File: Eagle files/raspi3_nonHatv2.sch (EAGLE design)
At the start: 37 parts, among them IC5 PAM8403, K1 PIN20X2

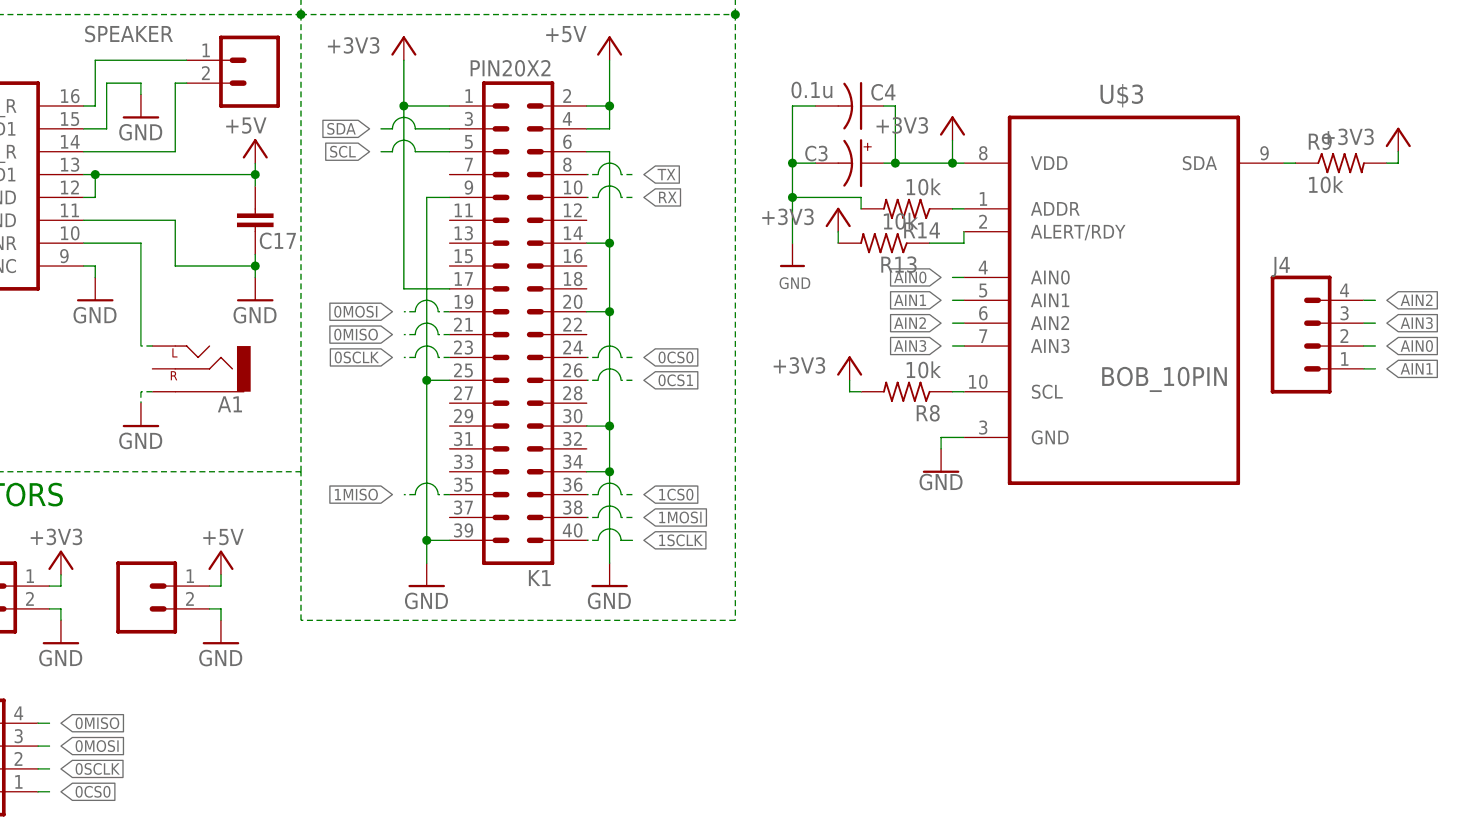
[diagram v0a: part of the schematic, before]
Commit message: rearranged
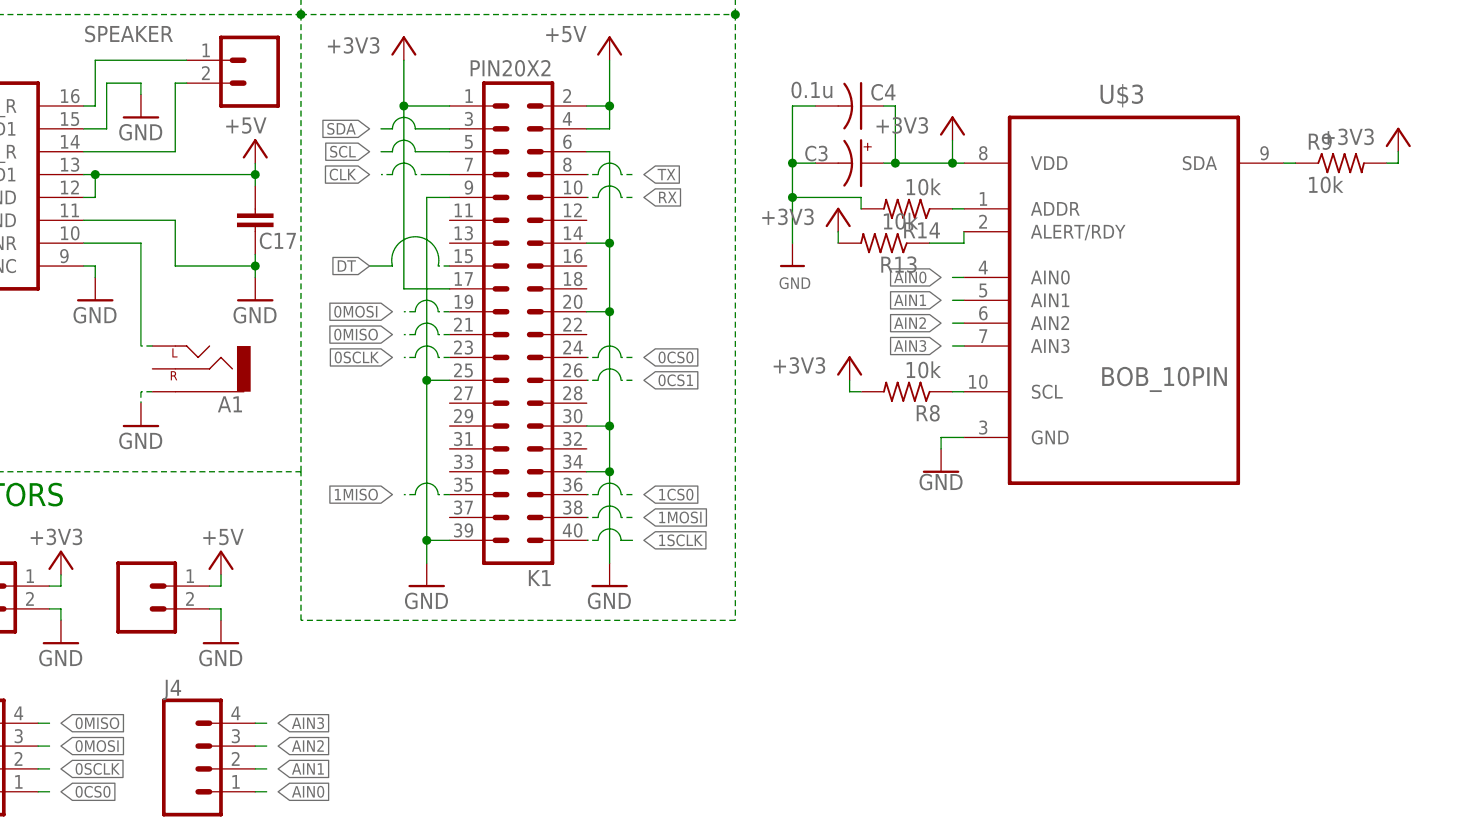
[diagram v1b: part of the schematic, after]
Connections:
- net AIN0: now also J4.1; no longer J4.2
- net AIN1: now also J4.2; no longer J4.1
- net AIN2: now also J4.3; no longer J4.4
- net AIN3: now also J4.4; no longer J4.3
- net CLK: now also K1.7
- net DT: now also K1.15
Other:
- moved on the sheet: J4
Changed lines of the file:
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@@
 <?xml version="1.0" encoding="utf-8"?>
 <!DOCTYPE eagle SYSTEM "eagle.dtd">
-<eagle version="9.6.2">
+<eagle version="9.4.1">
 <drawing>
 <settings>
@@
 <attribute name="NAME" x="-19.05" y="5.588" size="1.778" layer="95" font="vector"/>
 </instance>
-<instance part="J4" gate="G$1" x="133.35" y="44.45" smashed="yes">
-<attribute name="VALUE" x="128.27" y="37.084" size="1.778" layer="96" font="vector"/>
-<attribute name="NAME" x="128.27" y="52.578" size="1.778" layer="95" font="vector"/>
+<instance part="J4" gate="G$1" x="10.16" y="-2.54" smashed="yes">
+<attribute name="VALUE" x="5.08" y="-9.906" size="1.778" layer="96" font="vector"/>
+<attribute name="NAME" x="5.08" y="5.588" size="1.778" layer="95" font="vector"/>
 </instance>
 <instance part="U$3" gate="G$1" x="111.76" y="49.53" smashed="yes">
@@
 <label x="-34.29" y="119.38" size="1.27" layer="95" font="vector" ratio="17" rot="R90" xref="yes"/>
 </segment>
+<segment>
+<wire x1="36.83" y1="53.34" x2="35.56" y2="53.34" width="0.1524" layer="91" style="dashdot"/>
+<pinref part="K1" gate="G$1" pin="15"/>
+<wire x1="35.56" y1="53.34" x2="30.48" y2="53.34" width="0.1524" layer="91" curve="208.072487"/>
+<wire x1="30.48" y1="53.34" x2="27.94" y2="53.34" width="0.1524" layer="91"/>
+<label x="27.94" y="53.34" size="1.27" layer="95" font="vector" ratio="16" rot="R180" xref="yes"/>
+</segment>
 </net>
 <net name="CLK" class="0">
@@
 <wire x1="-41.91" y1="118.11" x2="-41.91" y2="115.57" width="0.1524" layer="91"/>
 <label x="-41.91" y="119.38" size="1.27" layer="95" font="vector" ratio="17" rot="R90" xref="yes"/>
+</segment>
+<segment>
+<wire x1="34.29" y1="63.5" x2="33.02" y2="63.5" width="0.1524" layer="91" style="dashdot"/>
+<wire x1="33.02" y1="63.5" x2="30.48" y2="63.5" width="0.1524" layer="91" curve="180"/>
+<wire x1="30.48" y1="63.5" x2="29.21" y2="63.5" width="0.1524" layer="91" style="dashdot"/>
+<pinref part="K1" gate="G$1" pin="7"/>
+<wire x1="36.83" y1="63.5" x2="34.29" y2="63.5" width="0.1524" layer="91"/>
+<label x="27.94" y="63.5" size="1.27" layer="95" font="vector" ratio="16" rot="R180" xref="yes"/>
 </segment>
 </net>
@@
 </segment>
 <segment>
-<pinref part="J4" gate="G$1" pin="2"/>
-<wire x1="138.43" y1="44.45" x2="139.7" y2="44.45" width="0.1524" layer="91"/>
-<label x="140.97" y="44.45" size="1.27" layer="95" font="vector" ratio="16" xref="yes"/>
+<pinref part="J4" gate="G$1" pin="1"/>
+<wire x1="15.24" y1="-5.08" x2="16.51" y2="-5.08" width="0.1524" layer="91"/>
+<label x="17.78" y="-5.08" size="1.27" layer="95" font="vector" ratio="16" xref="yes"/>
 </segment>
 </net>
@@
 </segment>
 <segment>
-<pinref part="J4" gate="G$1" pin="1"/>
-<wire x1="138.43" y1="41.91" x2="139.7" y2="41.91" width="0.1524" layer="91"/>
-<label x="140.97" y="41.91" size="1.27" layer="95" font="vector" ratio="16" xref="yes"/>
+<pinref part="J4" gate="G$1" pin="2"/>
+<wire x1="15.24" y1="-2.54" x2="16.51" y2="-2.54" width="0.1524" layer="91"/>
+<label x="17.78" y="-2.54" size="1.27" layer="95" font="vector" ratio="16" xref="yes"/>
 </segment>
 </net>
@@
 </segment>
 <segment>
-<pinref part="J4" gate="G$1" pin="4"/>
-<wire x1="138.43" y1="49.53" x2="139.7" y2="49.53" width="0.1524" layer="91"/>
-<label x="140.97" y="49.53" size="1.27" layer="95" font="vector" ratio="16" xref="yes"/>
+<pinref part="J4" gate="G$1" pin="3"/>
+<wire x1="15.24" y1="0" x2="16.51" y2="0" width="0.1524" layer="91"/>
+<label x="17.78" y="0" size="1.27" layer="95" font="vector" ratio="16" xref="yes"/>
 </segment>
 </net>
@@
 </segment>
 <segment>
-<pinref part="J4" gate="G$1" pin="3"/>
-<wire x1="138.43" y1="46.99" x2="139.7" y2="46.99" width="0.1524" layer="91"/>
-<label x="140.97" y="46.99" size="1.27" layer="95" font="vector" ratio="16" xref="yes"/>
-</segment>
-</net>
+<pinref part="J4" gate="G$1" pin="4"/>
+<wire x1="15.24" y1="2.54" x2="16.51" y2="2.54" width="0.1524" layer="91"/>
+<label x="17.78" y="2.54" size="1.27" layer="95" font="vector" ratio="16" xref="yes"/>
+</segment>
+</net>

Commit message: restored v4
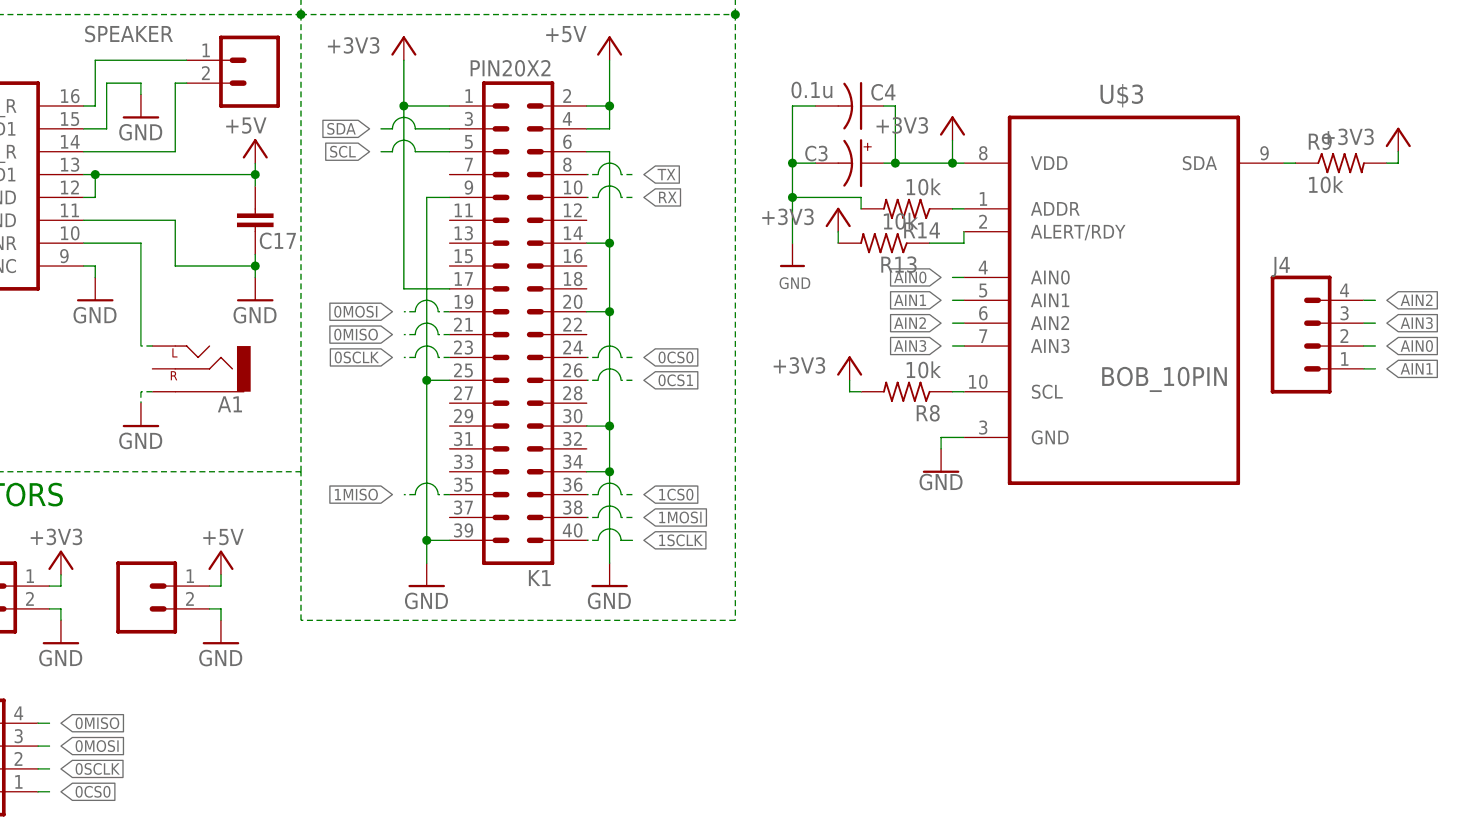
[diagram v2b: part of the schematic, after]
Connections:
- net AIN0: now also J4.2; no longer J4.1
- net AIN1: now also J4.1; no longer J4.2
- net AIN2: now also J4.4; no longer J4.3
- net AIN3: now also J4.3; no longer J4.4
- net CLK: no longer K1.7
- net DT: no longer K1.15
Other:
- moved on the sheet: J4
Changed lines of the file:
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@@
 <?xml version="1.0" encoding="utf-8"?>
 <!DOCTYPE eagle SYSTEM "eagle.dtd">
-<eagle version="9.4.1">
+<eagle version="9.6.2">
 <drawing>
 <settings>
@@
 <attribute name="NAME" x="-19.05" y="5.588" size="1.778" layer="95" font="vector"/>
 </instance>
-<instance part="J4" gate="G$1" x="10.16" y="-2.54" smashed="yes">
-<attribute name="VALUE" x="5.08" y="-9.906" size="1.778" layer="96" font="vector"/>
-<attribute name="NAME" x="5.08" y="5.588" size="1.778" layer="95" font="vector"/>
+<instance part="J4" gate="G$1" x="133.35" y="44.45" smashed="yes">
+<attribute name="VALUE" x="128.27" y="37.084" size="1.778" layer="96" font="vector"/>
+<attribute name="NAME" x="128.27" y="52.578" size="1.778" layer="95" font="vector"/>
 </instance>
 <instance part="U$3" gate="G$1" x="111.76" y="49.53" smashed="yes">
@@
 <label x="-34.29" y="119.38" size="1.27" layer="95" font="vector" ratio="17" rot="R90" xref="yes"/>
 </segment>
-<segment>
-<wire x1="36.83" y1="53.34" x2="35.56" y2="53.34" width="0.1524" layer="91" style="dashdot"/>
-<pinref part="K1" gate="G$1" pin="15"/>
-<wire x1="35.56" y1="53.34" x2="30.48" y2="53.34" width="0.1524" layer="91" curve="208.072487"/>
-<wire x1="30.48" y1="53.34" x2="27.94" y2="53.34" width="0.1524" layer="91"/>
-<label x="27.94" y="53.34" size="1.27" layer="95" font="vector" ratio="16" rot="R180" xref="yes"/>
-</segment>
 </net>
 <net name="CLK" class="0">
@@
 <wire x1="-41.91" y1="118.11" x2="-41.91" y2="115.57" width="0.1524" layer="91"/>
 <label x="-41.91" y="119.38" size="1.27" layer="95" font="vector" ratio="17" rot="R90" xref="yes"/>
-</segment>
-<segment>
-<wire x1="34.29" y1="63.5" x2="33.02" y2="63.5" width="0.1524" layer="91" style="dashdot"/>
-<wire x1="33.02" y1="63.5" x2="30.48" y2="63.5" width="0.1524" layer="91" curve="180"/>
-<wire x1="30.48" y1="63.5" x2="29.21" y2="63.5" width="0.1524" layer="91" style="dashdot"/>
-<pinref part="K1" gate="G$1" pin="7"/>
-<wire x1="36.83" y1="63.5" x2="34.29" y2="63.5" width="0.1524" layer="91"/>
-<label x="27.94" y="63.5" size="1.27" layer="95" font="vector" ratio="16" rot="R180" xref="yes"/>
 </segment>
 </net>
@@
 </segment>
 <segment>
-<pinref part="J4" gate="G$1" pin="1"/>
-<wire x1="15.24" y1="-5.08" x2="16.51" y2="-5.08" width="0.1524" layer="91"/>
-<label x="17.78" y="-5.08" size="1.27" layer="95" font="vector" ratio="16" xref="yes"/>
+<pinref part="J4" gate="G$1" pin="2"/>
+<wire x1="138.43" y1="44.45" x2="139.7" y2="44.45" width="0.1524" layer="91"/>
+<label x="140.97" y="44.45" size="1.27" layer="95" font="vector" ratio="16" xref="yes"/>
 </segment>
 </net>
@@
 </segment>
 <segment>
-<pinref part="J4" gate="G$1" pin="2"/>
-<wire x1="15.24" y1="-2.54" x2="16.51" y2="-2.54" width="0.1524" layer="91"/>
-<label x="17.78" y="-2.54" size="1.27" layer="95" font="vector" ratio="16" xref="yes"/>
+<pinref part="J4" gate="G$1" pin="1"/>
+<wire x1="138.43" y1="41.91" x2="139.7" y2="41.91" width="0.1524" layer="91"/>
+<label x="140.97" y="41.91" size="1.27" layer="95" font="vector" ratio="16" xref="yes"/>
 </segment>
 </net>
@@
 </segment>
 <segment>
-<pinref part="J4" gate="G$1" pin="3"/>
-<wire x1="15.24" y1="0" x2="16.51" y2="0" width="0.1524" layer="91"/>
-<label x="17.78" y="0" size="1.27" layer="95" font="vector" ratio="16" xref="yes"/>
+<pinref part="J4" gate="G$1" pin="4"/>
+<wire x1="138.43" y1="49.53" x2="139.7" y2="49.53" width="0.1524" layer="91"/>
+<label x="140.97" y="49.53" size="1.27" layer="95" font="vector" ratio="16" xref="yes"/>
 </segment>
 </net>
@@
 </segment>
 <segment>
-<pinref part="J4" gate="G$1" pin="4"/>
-<wire x1="15.24" y1="2.54" x2="16.51" y2="2.54" width="0.1524" layer="91"/>
-<label x="17.78" y="2.54" size="1.27" layer="95" font="vector" ratio="16" xref="yes"/>
-</segment>
-</net>
+<pinref part="J4" gate="G$1" pin="3"/>
+<wire x1="138.43" y1="46.99" x2="139.7" y2="46.99" width="0.1524" layer="91"/>
+<label x="140.97" y="46.99" size="1.27" layer="95" font="vector" ratio="16" xref="yes"/>
+</segment>
+</net>
